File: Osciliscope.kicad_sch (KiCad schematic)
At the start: 25 parts, among them J1 U.FL, J2 Conn_01x04_Socket, J3 U.FL, J4 Conn_01x04_Socket, SW1 SW_Rotary_1x8_MP, SW2 SW_Rotary_1x8_MP, U1 MCP1700x-330xxMB, U2 ADC082S101, U5 TLV9061xDBV, U7 TLV9061xDBV, U8 MCP4251-104E/ML-ND

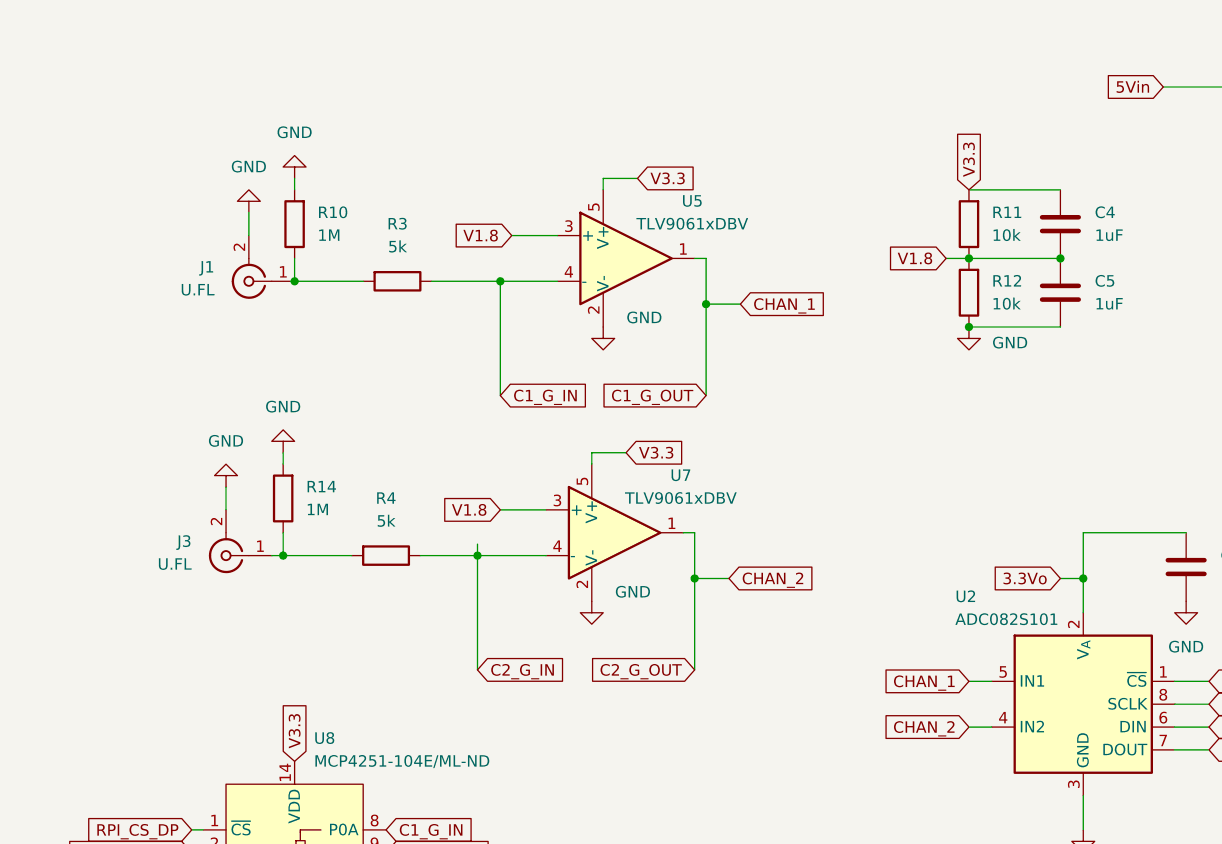
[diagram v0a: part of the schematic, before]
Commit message: PCB design
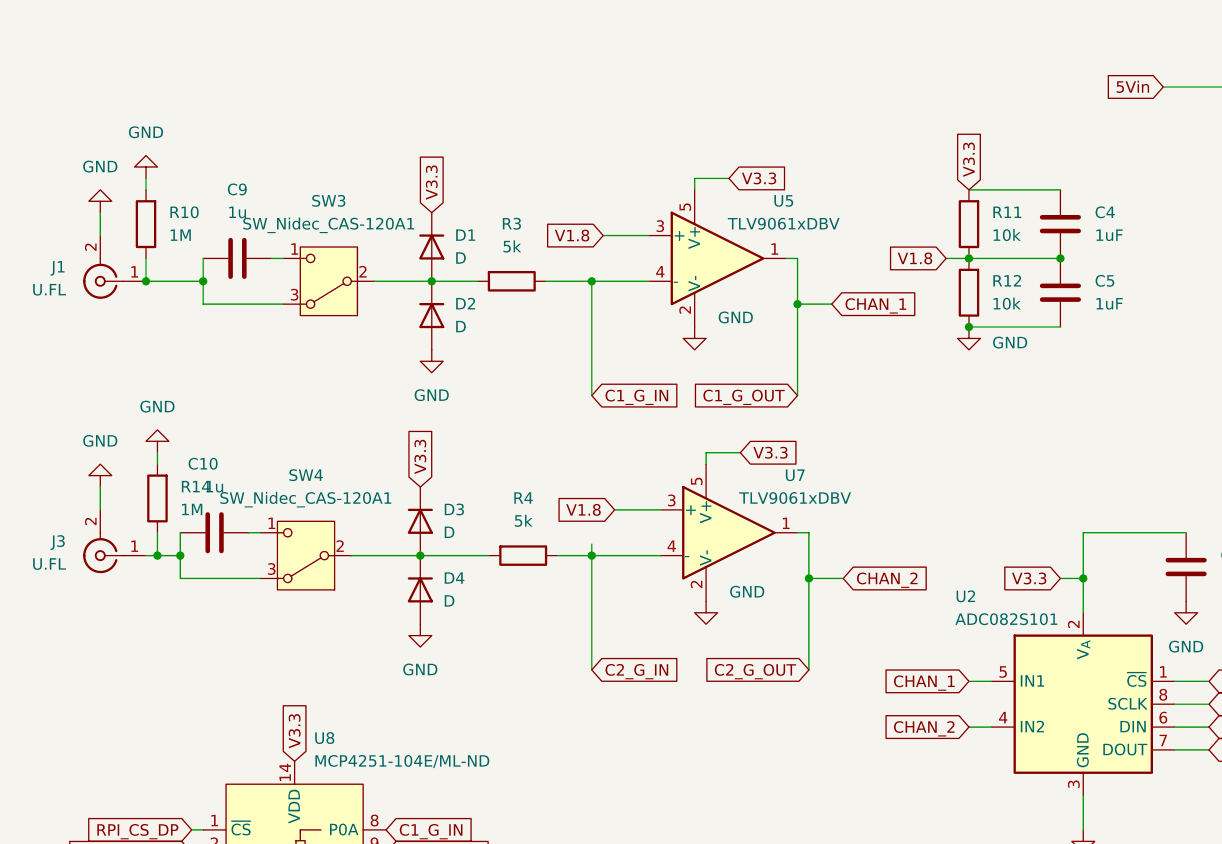
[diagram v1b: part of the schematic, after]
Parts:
- added C10, C9: 1u, Capacitor_SMD:C_1206_3216Metric, symbol Device:C
- added D1, D2, D3, D4: D, Diode_SMD:D_0201_0603Metric, symbol Device:D
- added SW3, SW4: SW_Nidec_CAS-120A1, Button_Switch_SMD:Nidec_Copal_CAS-120A, symbol Switch:SW_Nidec_CAS-120A1
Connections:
- net 3.3Vo is gone; now on net V3.3: C3.1, U2.2 (V_{A})
- net GND: now also D2.2 (A), D4.2 (A)
- net V3.3: now also D1.1 (K), D3.1 (K)
- net at J1.1 (In), R10.1: now also C9.1, SW3.3 (A); no longer R3.2
- net at J3.1 (In), R14.1: now also C10.1, SW4.3 (A); no longer R4.2
- new net: D3.2 (A), D4.1 (K), R4.2, SW4.2 (B)
- new net: C10.2, SW4.1 (C)
- new net: D1.2 (A), D2.1 (K), R3.2, SW3.2 (B)
- new net: C9.2, SW3.1 (C)
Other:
- moved on the sheet: J1, J3, R10, R14, R3, R4, U5, U7

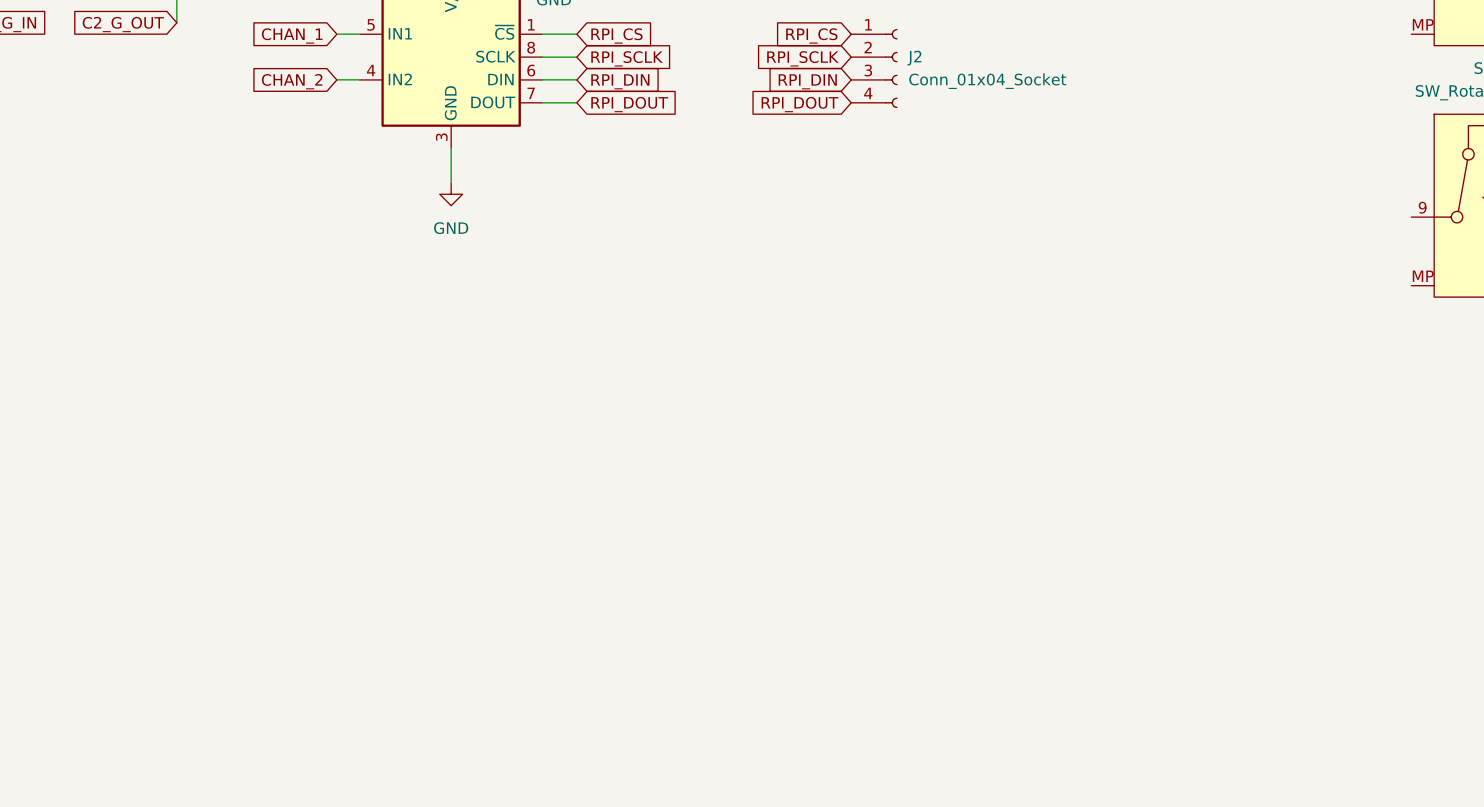
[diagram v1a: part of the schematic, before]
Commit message: USBC PD
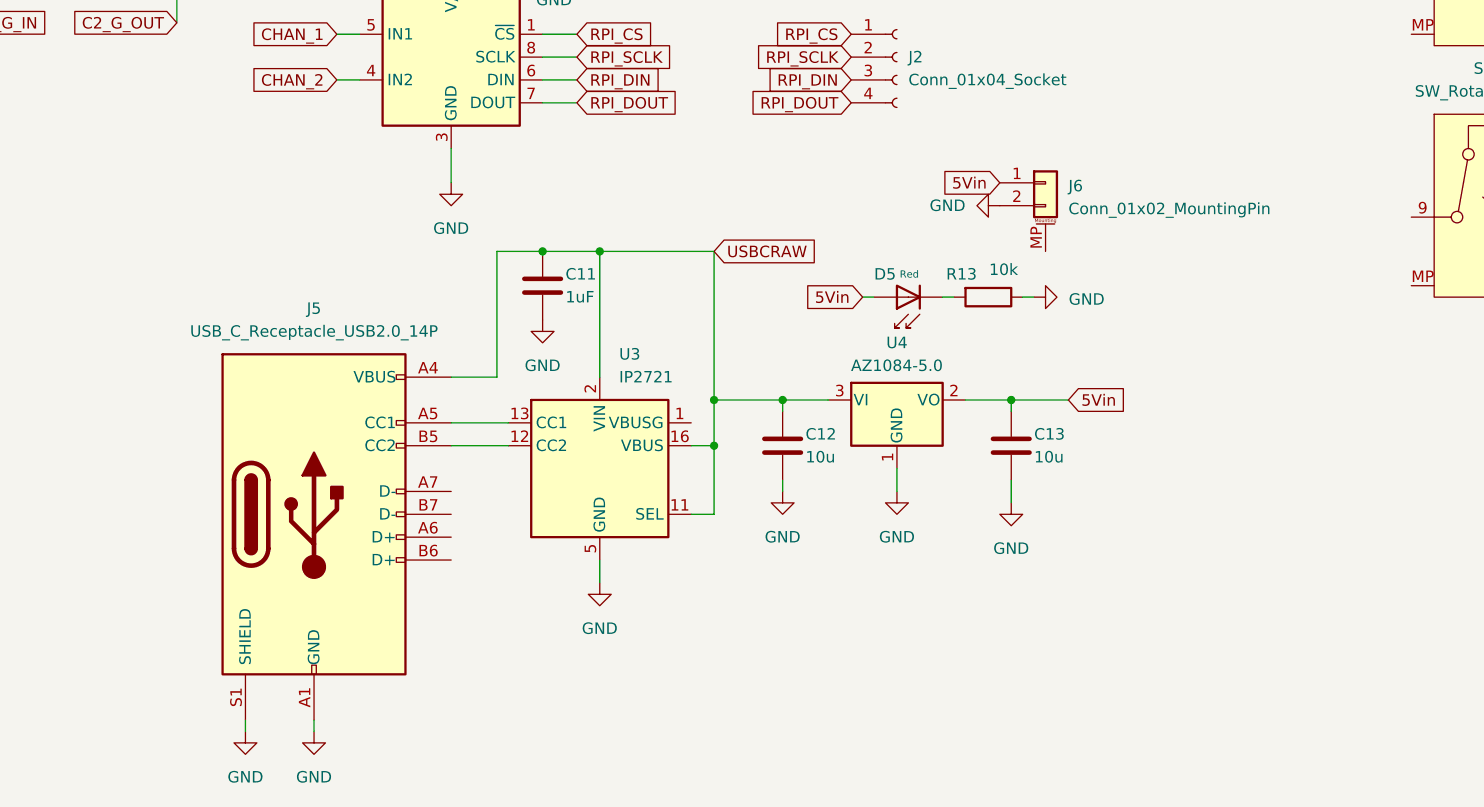
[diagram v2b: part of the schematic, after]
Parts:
- added C11: 1uF, Capacitor_SMD:C_1206_3216Metric, symbol Device:C
- added C12, C13: 10u, Capacitor_SMD:C_1206_3216Metric, symbol Device:C
- added D5: Red, PCM_JLCPCB:D_0805, symbol PCM_JLCPCB-Diodes:LED,0805,Red
- added J5: USB_C_Receptacle_USB2.0_14P, Connector_USB:USB_C_Receptacle_Amphenol_124019772112A, symbol Connector:USB_C_Receptacle_USB2.0_14P
- added J6: Conn_01x02_MountingPin, symbol Connector_Generic_MountingPin:Conn_01x02_MountingPin
- added R13: 10k, Capacitor_SMD:C_0603_1608Metric, symbol Device:R
- added U3: IP2721, Package_SO:TSSOP-16_4.4x5mm_P0.65mm, symbol Interface_USB:IP2721
- added U4: AZ1084-5.0, Package_TO_SOT_SMD:TO-252-2, symbol Regulator_Linear:AZ1084-5.0
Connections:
- net 5Vin: now also C13.1, D5.2, J6.1 (Pin_1), U4.2 (VO)
- net GND: now also C11.2, C12.2, C13.2, J5.A1 (GND), J5.A12 (GND), J5.B1 (GND), J5.B12 (GND), J5.S1 (SHIELD), J6.2 (Pin_2), R13.1, U3.5 (GND), U4.1 (GND)
- new net: J5.A5 (CC1), U3.13 (CC1)
- new net: J5.B5 (CC2), U3.12 (CC2)
- new net: D5.1, R13.2
- new net USBCRAW: C11.1, C12.1, J5.A4 (VBUS), J5.A9 (VBUS), J5.B4 (VBUS), J5.B9 (VBUS), U3.11 (SEL), U3.16 (VBUS), U3.2 (VIN), U4.3 (VI)
